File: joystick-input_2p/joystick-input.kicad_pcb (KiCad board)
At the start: 2 copper layers, 53.3 x 39.9 mm, 17 parts, among them J1 Conn_01x18, J2 Conn_02x14_Odd_Even

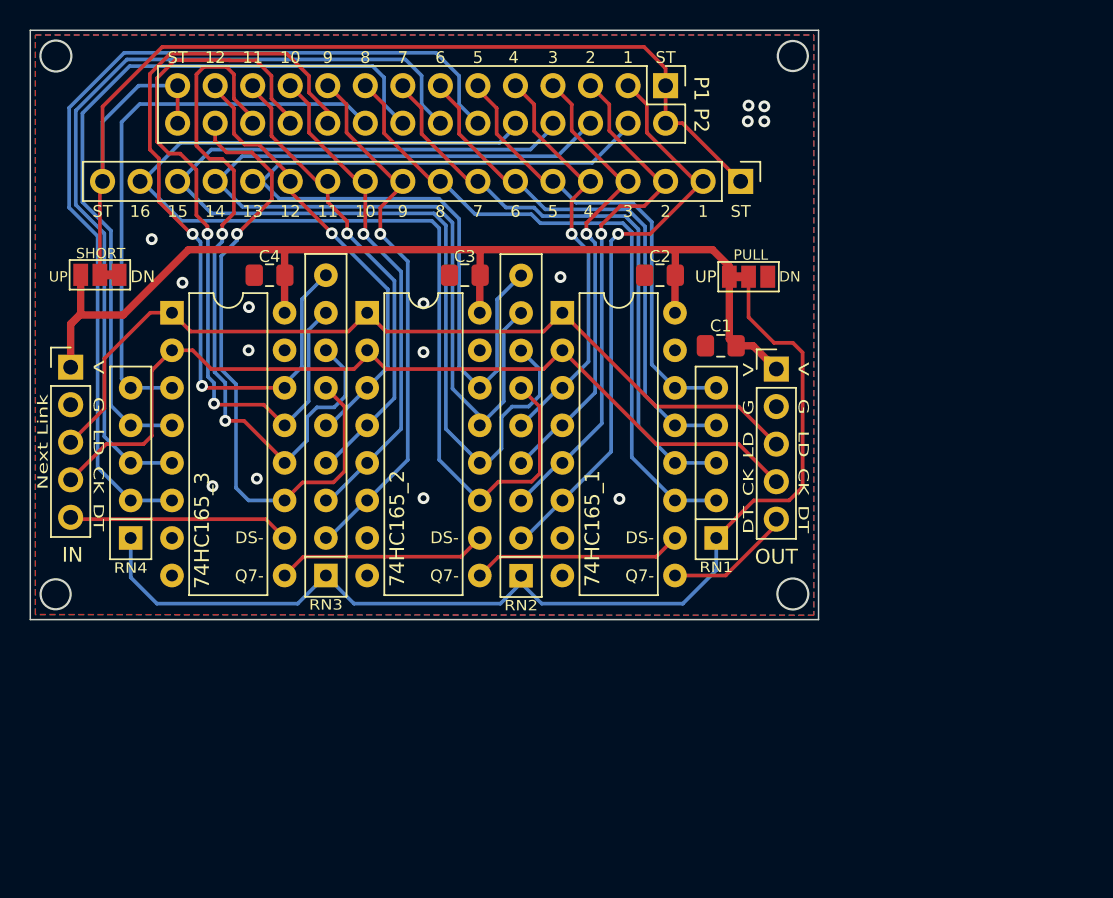
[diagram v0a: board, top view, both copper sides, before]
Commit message: 도면 시트 설명 추가
Signed-off-by: Ju, Gyeong-min <jcmh74@gmail.com>
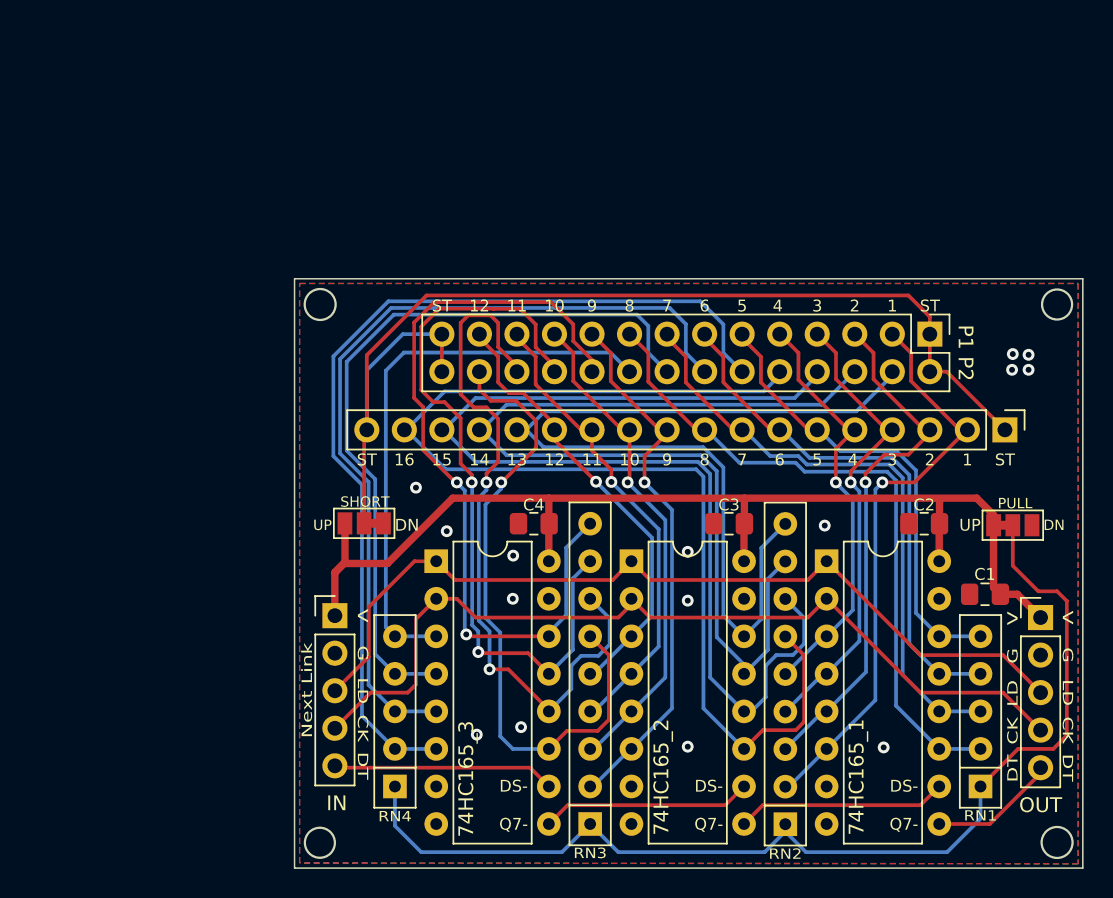
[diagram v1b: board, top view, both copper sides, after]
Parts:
- moved C1 24.5 mm to (176.4, 105.9)
- moved RN2 24.5 mm to (162.9, 121.5)
- moved RN3 24.5 mm to (149.7, 121.5)
- moved C2 24.5 mm to (172.3, 101.1)
- moved C3 24.5 mm to (159.1, 101.1)
- moved C4 24.5 mm to (145.9, 101.1)
- moved J2 24.5 mm to (172.7, 88.3)
- moved RN1 24.5 mm to (176.1, 118.9)
- moved 74HC165_1 24.5 mm to (165.7, 103.7)
- moved 74HC165_2 24.5 mm to (152.5, 103.7)
- moved 74HC165_3 24.5 mm to (139.3, 103.7)
- moved J1 24.5 mm to (177.8, 94.8)
- moved OUT1 24.5 mm to (180.2, 107.5)
- moved PULL1 24.5 mm to (178.3, 101.2)
- moved SHORT1 24.5 mm to (134.4, 101.1)
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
